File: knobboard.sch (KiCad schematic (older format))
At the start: 0 parts

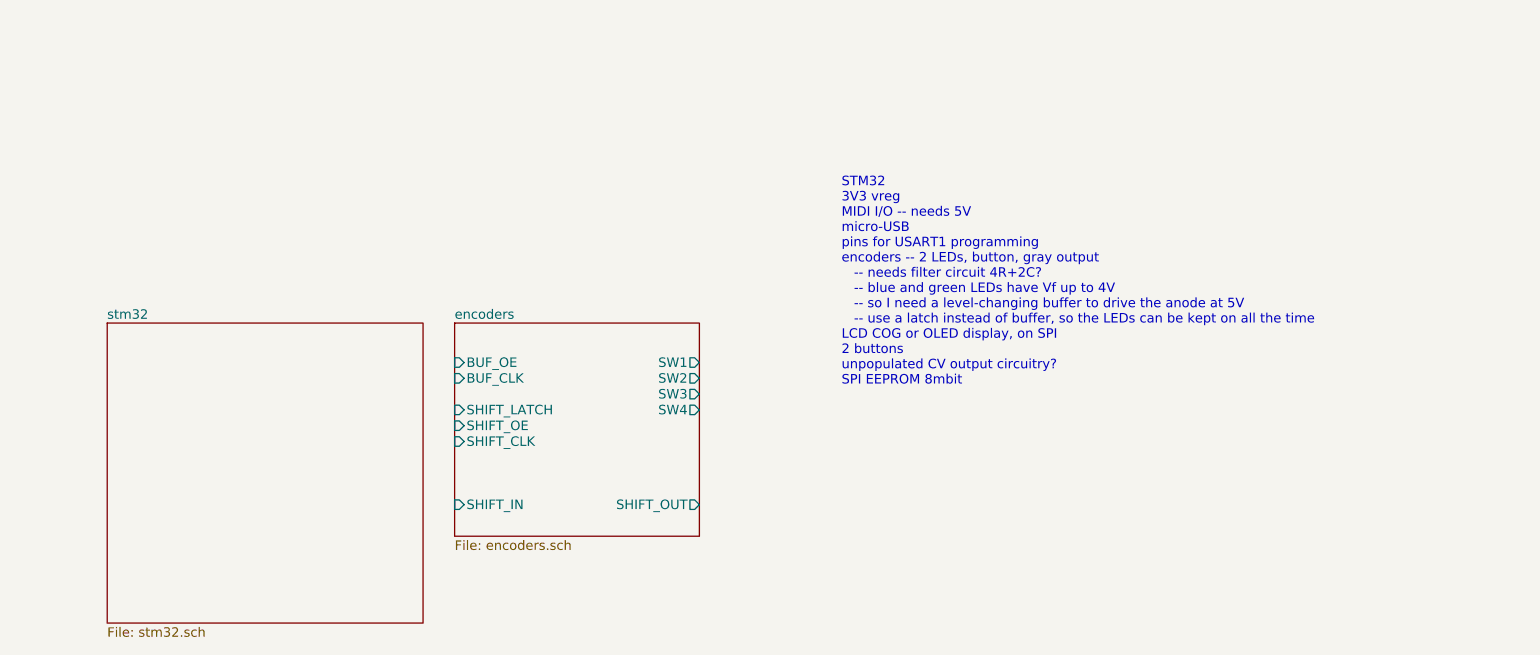
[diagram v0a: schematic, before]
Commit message: updates.
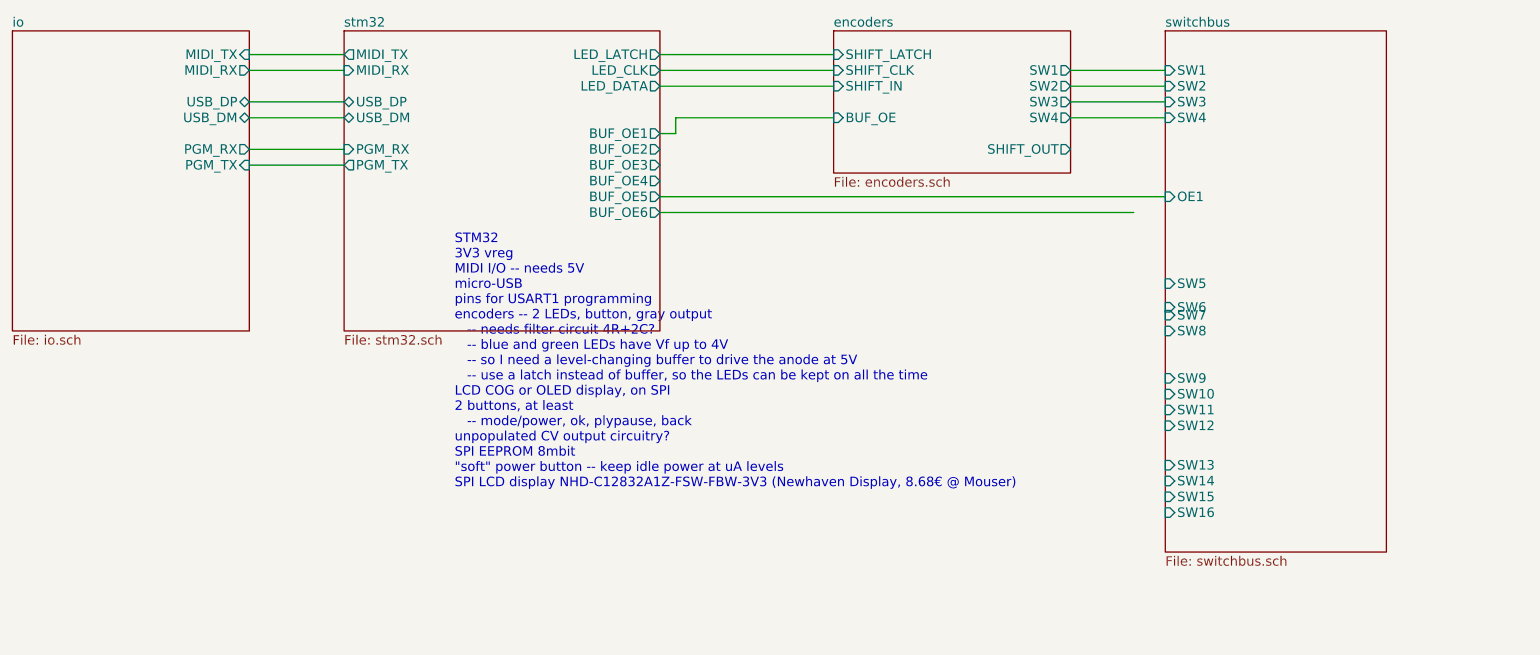
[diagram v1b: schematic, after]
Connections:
- wire segments 0 -> 18
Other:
- note added: "STM32\n3V3 vreg\nMIDI I/O -- needs 5V\nmicro-USB\npins for USART1 programming\nencoders -- 2 LEDs, button, gray output\n -- needs filter circuit 4R+2C?\n -- blue and green LEDs have Vf up to 4V\n -- so I need a level-changing buffer to drive the anode at 5V\n -- use a latch instead of buffer, so the LEDs can be kept on all the time\nLCD COG or OLED display, on SPI\n2 buttons, at least\n -- mode/p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"
- note removed: "STM32\n3V3 vreg\nMIDI I/O -- needs 5V\nmicro-USB\npins for USART1 programming\nencoders -- 2 LEDs, button, gray output\n -- needs filter circuit 4R+2C?\n -- blue and green LEDs have Vf up to 4V\n -- so I need a level-changing buffer to drive the anode at 5V\n -- use a latch instead of buffer, so the LEDs can be kept on all the time\nLCD COG or OLED display, on SPI\n2 buttons\nunpopulated CV outpu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"
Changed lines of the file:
@@
-EESchema Schematic File Version 2  date Fri 06 Apr 2012 09:44:16 PM CEST
+EESchema Schematic File Version 2  date Sun 08 Apr 2012 06:37:26 PM CEST
 LIBS:power
 LIBS:device
@@
 LIBS:bourns-encoder
 LIBS:stm32
+LIBS:spi-flash
+LIBS:nhd-lcd
+LIBS:r-network
 LIBS:knobboard-cache
 EELAYER 25  0
@@
 $Descr A4 11700 8267
 encoding utf-8
-Sheet 1 3
+Sheet 1 5
 Title ""
-Date "6 apr 2012"
+Date "8 apr 2012"
 Rev ""
 Comp ""
@@
 Comment4 ""
 $EndDescr
+Wire Wire Line
+	8800 2600 5600 2600
+Wire Wire Line
+	8200 1900 8800 1900
+Wire Wire Line
+	8200 2100 8800 2100
+Wire Wire Line
+	3000 2300 3600 2300
+Wire Wire Line
+	3000 2000 3600 2000
+Wire Wire Line
+	3000 1700 3600 1700
+Wire Wire Line
+	5600 1900 6700 1900
+Wire Wire Line
+	5600 1700 6700 1700
+Wire Wire Line
+	5600 1800 6700 1800
+Wire Wire Line
+	5600 2200 5700 2200
+Wire Wire Line
+	5700 2200 5700 2100
+Wire Wire Line
+	5700 2100 6700 2100
+Wire Wire Line
+	3600 1800 3000 1800
+Wire Wire Line
+	3600 2100 3000 2100
+Wire Wire Line
+	3600 2400 3000 2400
+Wire Wire Line
+	5600 2700 8600 2700
+Wire Wire Line
+	8200 2000 8800 2000
+Wire Wire Line
+	8200 1800 8800 1800
 $Sheet
-S 2100 3400 2000 1900
+S 8800 1550 1400 3300
+U 4F81A858
+F0 "switchbus" 60
+F1 "switchbus.sch" 60
+F2 "OE1" I L 8800 2600 60
+F3 "SW16" I L 8800 4600 60
+F4 "SW15" I L 8800 4500 60
+F5 "SW14" I L 8800 4400 60
+F6 "SW13" I L 8800 4300 60
+F7 "SW12" I L 8800 4050 60
+F8 "SW11" I L 8800 3950 60
+F9 "SW10" I L 8800 3850 60
+F10 "SW9" I L 8800 3750 60
+F11 "SW8" I L 8800 3450 60
+F12 "SW7" I L 8800 3350 60
+F13 "SW6" I L 8800 3300 60
+F14 "SW5" I L 8800 3150 60
+F15 "SW4" I L 8800 2100 60
+F16 "SW3" I L 8800 2000 60
+F17 "SW2" I L 8800 1900 60
+F18 "SW1" I L 8800 1800 60
+$EndSheet
+$Sheet
+S 1500 1550 1500 1900
+U 4F80537C
+F0 "io" 60
+F1 "io.sch" 60
+F2 "MIDI_RX" O R 3000 1800 60
+F3 "MIDI_TX" I R 3000 1700 60
+F4 "PGM_TX" I R 3000 2400 60
+F5 "PGM_RX" O R 3000 2300 60
+F6 "USB_DM" B R 3000 2100 60
+F7 "USB_DP" B R 3000 2000 60
+$EndSheet
+$Sheet
+S 3600 1550 2000 1900
 U 4F7EF61F
 F0 "stm32" 60
 F1 "stm32.sch" 60
+F2 "LED_LATCH" O R 5600 1700 60
+F3 "LED_DATA" O R 5600 1900 60
+F4 "LED_CLK" O R 5600 1800 60
+F5 "BUF_OE6" O R 5600 2700 60
+F6 "BUF_OE5" O R 5600 2600 60
+F7 "BUF_OE4" O R 5600 2500 60
+F8 "BUF_OE3" O R 5600 2400 60
+F9 "BUF_OE2" O R 5600 2300 60
+F10 "BUF_OE1" O R 5600 2200 60
+F11 "MIDI_TX" O L 3600 1700 60
+F12 "MIDI_RX" I L 3600 1800 60
+F13 "USB_DP" B L 3600 2000 60
+F14 "USB_DM" B L 3600 2100 60
+F15 "PGM_RX" I L 3600 2300 60
+F16 "PGM_TX" O L 3600 2400 60
 $EndSheet
 $Sheet
-S 4300 3400 1550 1350
+S 6700 1550 1500 900
 U 4F7E05A5
 F0 "encoders" 60
 F1 "encoders.sch" 60
-F2 "BUF_OE" I L 4300 3650 60
-F3 "BUF_CLK" I L 4300 3750 60
-F4 "SW4" O R 5850 3950 60
-F5 "SW3" O R 5850 3850 60
-F6 "SW2" O R 5850 3750 60
-F7 "SW1" O R 5850 3650 60
-F8 "SHIFT_LATCH" I L 4300 3950 60
-F9 "SHIFT_OE" I L 4300 4050 60
-F10 "SHIFT_CLK" I L 4300 4150 60
-F11 "SHIFT_OUT" O R 5850 4550 60
-F12 "SHIFT_IN" I L 4300 4550 60
+F2 "BUF_OE" I L 6700 2100 60
+F3 "SW4" O R 8200 2100 60
+F4 "SW3" O R 8200 2000 60
+F5 "SW2" O R 8200 1900 60
+F6 "SW1" O R 8200 1800 60
+F7 "SHIFT_LATCH" I L 6700 1700 60
+F8 "SHIFT_CLK" I L 6700 1800 60
+F9 "SHIFT_OUT" O R 8200 2300 60
+F10 "SHIFT_IN" I L 6700 1900 60
 $EndSheet
-Text Notes 6750 3800 0    60   ~ 0
-STM32\n3V3 vreg\nMIDI I/O -- needs 5V\nmicro-USB\npins for USART1 programming\nencoders -- 2 LEDs, button, gray output\n   -- needs filter circuit 4R+2C?\n   -- blue and green LEDs have Vf up to 4V\n   -- so I need a level-changing buffer to drive the anode at 5V\n   -- use a latch instead of buffer, so the LEDs can be kept on all the time\nLCD COG or OLED display, on SPI\n2 buttons\nunpopulated CV output circuitry?\nSPI EEPROM 8mbit
+Text Notes 4300 4450 0    60   ~ 0
+STM32\n3V3 vreg\nMIDI I/O -- needs 5V\nmicro-USB\npins for USART1 programming\nencoders -- 2 LEDs, button, gray output\n   -- needs filter circuit 4R+2C?\n   -- blue and green LEDs have Vf up to 4V\n   -- so I need a level-changing buffer to drive the anode at 5V\n   -- use a latch instead of buffer, so the LEDs can be kept on all the time\nLCD COG or OLED display, on SPI\n2 buttons, at least\n   -- mode/power, ok, plypause, back\nunpopulated CV output circuitry?\nSPI EEPROM 8mbit\n"soft" power button -- keep idle power at uA levels\nSPI LCD display NHD-C12832A1Z-FSW-FBW-3V3 (Newhaven Display, 8.68€ @ Mouser)
 $EndSCHEMATC
